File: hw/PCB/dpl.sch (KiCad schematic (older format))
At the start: 4 parts, among them U3 SN754410, U5 AV4524_2PIN

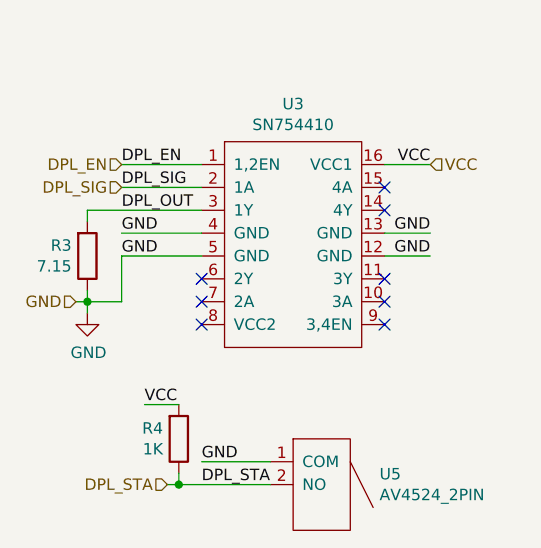
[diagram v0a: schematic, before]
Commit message: Finished preliminary design phase for the version 2.0.
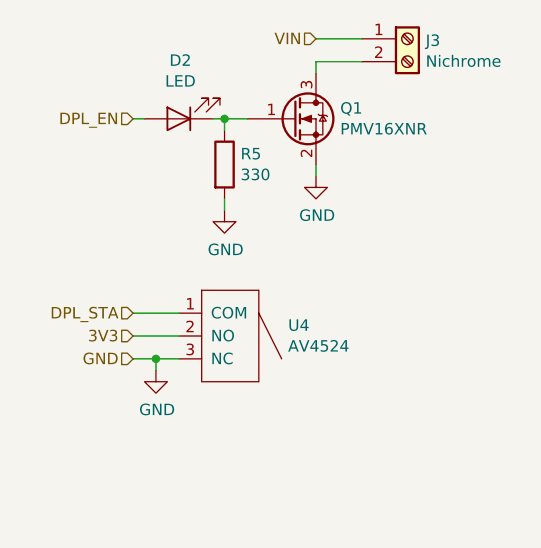
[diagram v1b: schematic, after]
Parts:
- removed R3: 7.15, Resistor_FOD:RCL12257R15FKEG, symbol Device:R
- removed R4: 1K, Resistor_SMD:R_0603_1608Metric_Pad1.05x0.95mm_HandSolder, symbol Device:R
- removed U3: SN754410, Package_DIP:DIP-16_W7.62mm, symbol H-Bridge:SN754410
- removed U5: AV4524_2PIN, Interrupt:AV4524_2PIN, symbol Interrupter:AV4524_2PIN
- added D2: LED, Diode_SMD:D_0805_2012Metric_Pad1.15x1.40mm_HandSolder, symbol Device:LED
- added J3: Nichrome, TerminalBlock:TerminalBlock_Altech_AK300-2_P5.00mm, symbol Connector:Screw_Terminal_01x02
- added Q1: PMV16XNR, Package_TO_SOT_SMD:SOT-23, symbol Transistor_FET:2N7002
- added R5: 330, Resistor_SMD:R_0603_1608Metric_Pad1.05x0.95mm_HandSolder, symbol Device:R
- added U4: AV4524, Interrupt:AV4524, symbol Interrupter:AV4524
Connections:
- net DPL_EN: now also D2.2 (A)
- net DPL_STA: now also U4.1 (COM)
- net GND: now also Q1.2 (S), R5.2, U4.3 (NC)
- new net: J3.2 (Pin_2), Q1.3 (D)
- new net: D2.1 (K), Q1.1 (G), R5.1
- new net 3V3: U4.2 (NO)
- new net VIN: J3.1 (Pin_1)
- no-connect marks 8 -> 0
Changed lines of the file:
@@
 EESchema Schematic File Version 5
-LIBS:FOD-cache
 EELAYER 29 0
 EELAYER END
 $Descr A4 11693 8268
 encoding utf-8
-Sheet 5 5
+Sheet 5 6
 Title ""
 Date ""
@@
 $EndDescr
 $Comp
-L H-Bridge:SN754410 U3
-U 1 1 5BEA29D2
-P 5650 3450
-F 0 "U3" H 5650 4065 50  0000 C CNN
-F 1 "SN754410" H 5650 3974 50  0000 C CNN
-F 2 "Package_DIP:DIP-16_W7.62mm" H 5500 3550 50  0001 C CNN
-F 3 "" H 5500 3550 50  0001 C CNN
-	1    5650 3450
+L power:GND #PWR0112
+U 1 1 5BEA3F1A
+P 5750 3150
+F 0 "#PWR0112" H 5750 2900 50  0001 C CNN
+F 1 "GND" H 5755 2977 50  0000 C CNN
+F 2 "" H 5750 3150 50  0001 C CNN
+F 3 "" H 5750 3150 50  0001 C CNN
+	1    5750 3150
+	1    0    0    -1
+$EndComp
+Text HLabel 4950 2900 0    50   Input ~ 0
+DPL_EN
+Text HLabel 4950 3950 0    50   Input ~ 0
+GND
+Text HLabel 5750 2550 0    50   Input ~ 0
+VIN
+Text HLabel 4950 3750 0    50   Input ~ 0
+DPL_STA
+$Comp
+L Connector:Screw_Terminal_01x02 J3
+U 1 1 5D23C1A6
+P 6150 2550
+F 0 "J3" H 6230 2542 50  0000 L CNN
+F 1 "Nichrome" H 6230 2451 50  0000 L CNN
+F 2 "TerminalBlock:TerminalBlock_Altech_AK300-2_P5.00mm" H 6150 2550 50  0001 C CNN
+F 3 "~" H 6150 2550 50  0001 C CNN
+	1    6150 2550
+	1    0    0    -1
+$EndComp
+Wire Wire Line
+	5750 2650 5750 2700
+Wire Wire Line
+	5750 2650 5950 2650
+Wire Wire Line
+	5950 2550 5750 2550
+Wire Wire Line
+	5750 3150 5750 3100
+$Comp
+L Interrupter:AV4524 U4
+U 1 1 5D23F1CD
+P 5350 3850
+F 0 "U4" H 5628 3896 50  0000 L CNN
+F 1 "AV4524" H 5628 3805 50  0000 L CNN
+F 2 "Interrupt:AV4524" H 5300 3850 50  0001 C CNN
+F 3 "" H 5300 3850 50  0001 C CNN
+	1    5350 3850
+	1    0    0    -1
+$EndComp
+Wire Wire Line
+	5150 3750 4950 3750
+Wire Wire Line
+	5150 3950 5050 3950
+Wire Wire Line
+	4950 3850 5150 3850
+Text HLabel 4950 3850 0    50   Input ~ 0
+3V3
+$Comp
+L power:GND #PWR0117
+U 1 1 5D2408D3
+P 5050 4000
+F 0 "#PWR0117" H 5050 3750 50  0001 C CNN
+F 1 "GND" H 5055 3827 50  0000 C CNN
+F 2 "" H 5050 4000 50  0001 C CNN
+F 3 "" H 5050 4000 50  0001 C CNN
+	1    5050 4000
+	1    0    0    -1
+$EndComp
+Wire Wire Line
+	5050 4000 5050 3950
+Connection ~ 5050 3950
+Wire Wire Line
+	5050 3950 4950 3950
+$Comp
+L Device:R R5
+U 1 1 5D23EA26
+P 5350 3100
+F 0 "R5" H 5420 3146 50  0000 L CNN
+F 1 "330" H 5420 3055 50  0000 L CNN
+F 2 "Resistor_SMD:R_0603_1608Metric_Pad1.05x0.95mm_HandSolder" V 5280 3100 50  0001 C CNN
+F 3 "~" H 5350 3100 50  0001 C CNN
+	1    5350 3100
 	1    0    0    -1
 $EndComp
 $Comp
-L Device:R R3
-U 1 1 5BEA225C
-P 4750 3500
-F 0 "R3" H 4681 3454 50  0000 R CNN
-F 1 "7.15" H 4681 3545 50  0000 R CNN
-F 2 "Resistor_FOD:RCL12257R15FKEG" V 4680 3500 50  0001 C CNN
-F 3 "~" H 4750 3500 50  0001 C CNN
-	1    4750 3500
-	1    0    0    1
+L Device:LED D2
+U 1 1 5D23EB22
+P 5150 2900
+F 0 "D2" H 5143 2645 50  0000 C CNN
+F 1 "LED" H 5143 2736 50  0000 C CNN
+F 2 "Diode_SMD:D_0805_2012Metric_Pad1.15x1.40mm_HandSolder" H 5150 2900 50  0001 C CNN
+F 3 "~" H 5150 2900 50  0001 C CNN
+	1    5150 2900
+	-1   0    0    1
 $EndComp
 Wire Wire Line
-	6050 3100 6250 3100
-Text Label 6250 3100 2    50   ~ 0
-VCC
-Text Label 4900 3200 0    50   ~ 0
-DPL_SIG
-Text Label 4900 3100 0    50   ~ 0
-DPL_EN
-Text Label 4900 3300 0    50   ~ 0
-DPL_OUT
+	5300 2900 5350 2900
 Wire Wire Line
-	5250 3100 4900 3100
+	5350 2900 5350 2950
 Wire Wire Line
-	4900 3200 5250 3200
-Wire Wire Line
-	5250 3400 4900 3400
-Wire Wire Line
-	4900 3500 5250 3500
-Wire Wire Line
-	6050 3400 6250 3400
-Wire Wire Line
-	6250 3500 6050 3500
-Text Label 4900 3400 0    50   ~ 0
-GND
-Text Label 4900 3500 0    50   ~ 0
-GND
-Text Label 6250 3400 2    50   ~ 0
-GND
-Text Label 6250 3500 2    50   ~ 0
-GND
-Wire Wire Line
-	4750 3300 4750 3350
-Wire Wire Line
-	4750 3300 5250 3300
-Wire Wire Line
-	4750 3650 4750 3700
-Wire Wire Line
-	4750 3700 4900 3700
-Wire Wire Line
-	4900 3700 4900 3500
-Wire Wire Line
-	4750 3700 4750 3750
-Connection ~ 4750 3700
+	5350 3250 5350 3300
 $Comp
-L power:GND #PWR0112
-U 1 1 5BEA3F1A
-P 4750 3750
-F 0 "#PWR0112" H 4750 3500 50  0001 C CNN
-F 1 "GND" H 4755 3577 50  0000 C CNN
-F 2 "" H 4750 3750 50  0001 C CNN
-F 3 "" H 4750 3750 50  0001 C CNN
-	1    4750 3750
+L power:GND #PWR0118
+U 1 1 5D23F136
+P 5350 3300
+F 0 "#PWR0118" H 5350 3050 50  0001 C CNN
+F 1 "GND" H 5355 3127 50  0000 C CNN
+F 2 "" H 5350 3300 50  0001 C CNN
+F 3 "" H 5350 3300 50  0001 C CNN
+	1    5350 3300
 	1    0    0    -1
 $EndComp
-Text HLabel 4900 3100 0    50   Input ~ 0
-DPL_EN
-Text HLabel 4900 3200 0    50   Input ~ 0
-DPL_SIG
-Text HLabel 4700 3700 0    50   Input ~ 0
-GND
 Wire Wire Line
-	4750 3700 4700 3700
-NoConn ~ 6050 3200
-NoConn ~ 6050 3300
-NoConn ~ 6050 3600
-NoConn ~ 6050 3700
-NoConn ~ 6050 3800
-NoConn ~ 5250 3600
-NoConn ~ 5250 3700
-NoConn ~ 5250 3800
-Text HLabel 6250 3100 2    50   Input ~ 0
-VCC
+	4950 2900 5000 2900
+Wire Wire Line
+	5350 2900 5450 2900
+Connection ~ 5350 2900
 $Comp
-L Device:R R4
-U 1 1 5BF60B18
-P 5150 4300
-F 0 "R4" H 5081 4254 50  0000 R CNN
-F 1 "1K" H 5081 4345 50  0000 R CNN
-F 2 "Resistor_SMD:R_0603_1608Metric_Pad1.05x0.95mm_HandSolder" V 5080 4300 50  0001 C CNN
-F 3 "~" H 5150 4300 50  0001 C CNN
-	1    5150 4300
-	1    0    0    1
-$EndComp
-Text Label 5250 4500 0    50   ~ 0
-DPL_STA
-Wire Wire Line
-	5250 4400 5550 4400
-Text Label 5250 4400 0    50   ~ 0
-GND
-Text Label 5000 4150 0    50   ~ 0
-VCC
-Wire Wire Line
-	5150 4150 5000 4150
-Wire Wire Line
-	5150 4500 5150 4450
-Wire Wire Line
-	5150 4500 5550 4500
-Wire Wire Line
-	5150 4500 5100 4500
-Connection ~ 5150 4500
-Text HLabel 5100 4500 0    50   Input ~ 0
-DPL_STA
-$Comp
-L Interrupter:AV4524_2PIN U5
-U 1 1 5BF65EF1
-P 5750 4500
-F 0 "U5" H 6028 4546 50  0000 L CNN
-F 1 "AV4524_2PIN" H 6028 4455 50  0000 L CNN
-F 2 "Interrupt:AV4524_2PIN" H 5700 4500 50  0001 C CNN
-F 3 "" H 5700 4500 50  0001 C CNN
-	1    5750 4500
+L Transistor_FET:2N7002 Q1
+U 1 1 5D257A79
+P 5650 2900
+F 0 "Q1" H 5856 2946 50  0000 L CNN
+F 1 "PMV16XNR" H 5856 2855 50  0000 L CNN
+F 2 "Package_TO_SOT_SMD:SOT-23" H 5850 2825 50  0001 L CIN
+F 3 "https://www.fairchildsemi.com/datasheets/2N/2N7002.pdf" H 5650 2900 50  0001 L CNN
+	1    5650 2900
 	1    0    0    -1
 $EndComp
